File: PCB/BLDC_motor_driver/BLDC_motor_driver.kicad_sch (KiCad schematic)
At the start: 4 parts, among them U2 AS5048A, U5 SN65HVD230, U6 STM32F405RGTx, U7 STM32F303K8Tx

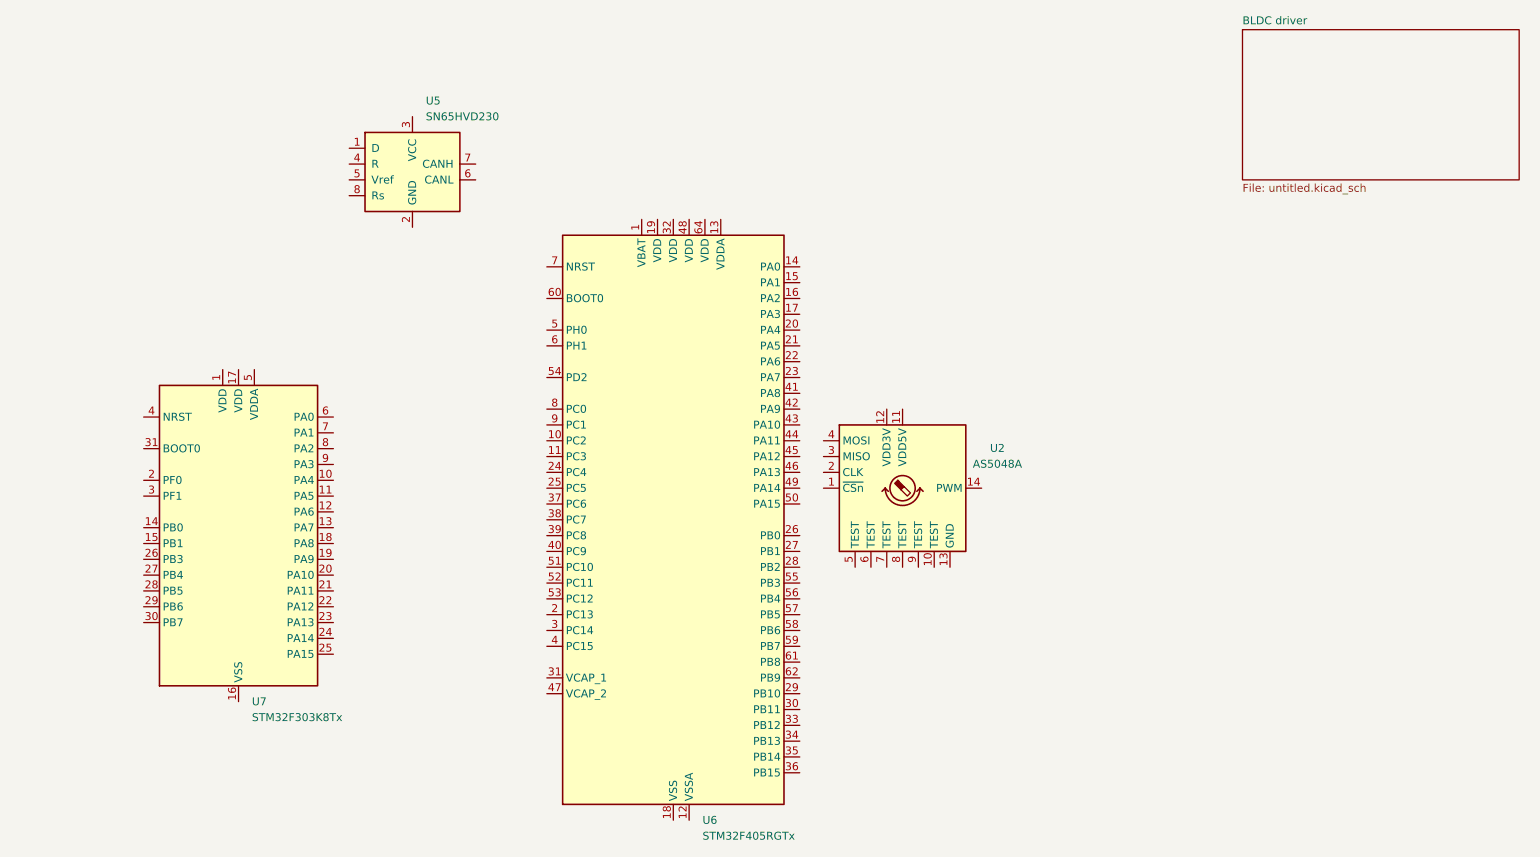
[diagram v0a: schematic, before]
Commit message: pcb progress
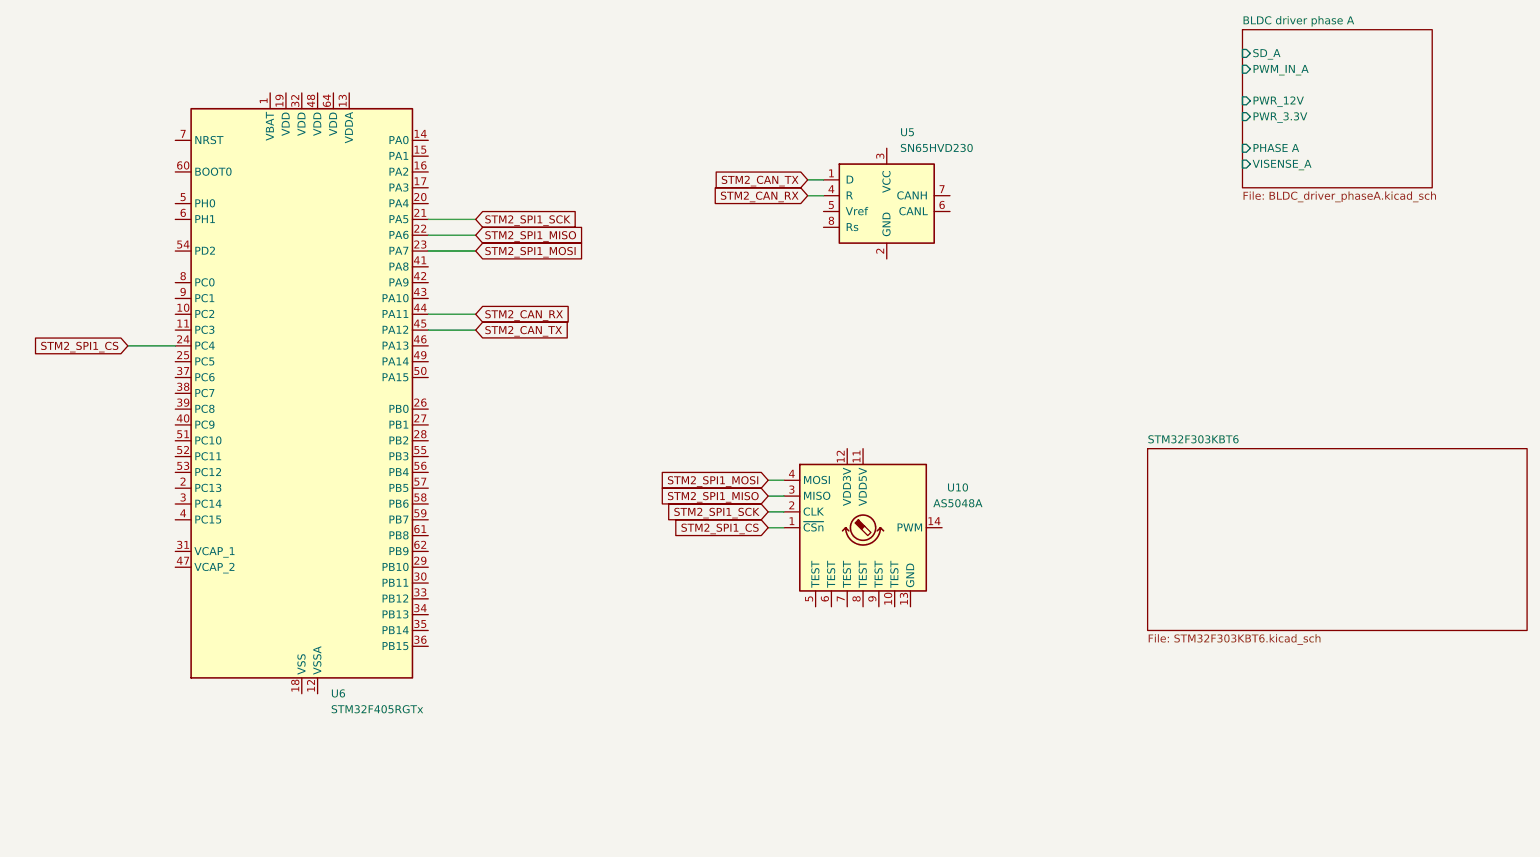
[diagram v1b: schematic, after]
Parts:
- removed U2: AS5048A, Package_SO:TSSOP-14_4.4x5mm_P0.65mm, symbol Sensor_Magnetic:AS5048A
- removed U7: STM32F303K8Tx, Package_QFP:LQFP-32_7x7mm_P0.8mm, symbol MCU_ST_STM32F3:STM32F303K8Tx
- added U10: AS5048A, Package_SO:TSSOP-14_4.4x5mm_P0.65mm, symbol Sensor_Magnetic:AS5048A
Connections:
- net STM2_CAN_TX: now reaches U5.1 (D)
- net STM2_CAN_TX: now also U6.45 (PA12)
- net STM2_CAN_RX: now reaches U5.4 (R)
- net STM2_CAN_RX: now also U6.44 (PA11)
- net STM2_SPI1_SCK: now reaches U6.21 (PA5)
- net STM2_SPI1_SCK: now also U10.2 (CLK)
- net STM2_SPI1_MISO: now reaches U6.22 (PA6)
- net STM2_SPI1_MISO: now also U10.3 (MISO)
- net STM2_SPI1_MOSI: now reaches U6.23 (PA7)
- net STM2_SPI1_MOSI: now also U10.4 (MOSI)
- net STM2_SPI1_CS: now reaches U6.24 (PC4)
- net STM2_SPI1_CS: now also U10.1 (~{CSn})
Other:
- sheet BLDC driver renamed BLDC driver phase A
- added sheet STM32F303KBT6 (STM32F303KBT6.kicad_sch)
- sheet BLDC driver phase A: file untitled.kicad_sch -> BLDC_driver_phaseA.kicad_sch
- sheet BLDC driver phase A ports: added PHASE A, PWM_IN_A, PWR_12V, PWR_3.3V, SD_A, VISENSE_A; removed none
- moved on the sheet: U5, U6
